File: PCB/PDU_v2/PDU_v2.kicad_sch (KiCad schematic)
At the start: 61 parts, among them J1 XT60PW-M, J14 Conn_01x04_Pin, J2 XT60PW-M, J3 XT60PW-M, J4 XT60PW-M, J5 XT60PW-M, J6 XT60PW-M, J7 XT60PW-M, U1 TPS54360BQDDAQ1, U2 INA240A2D

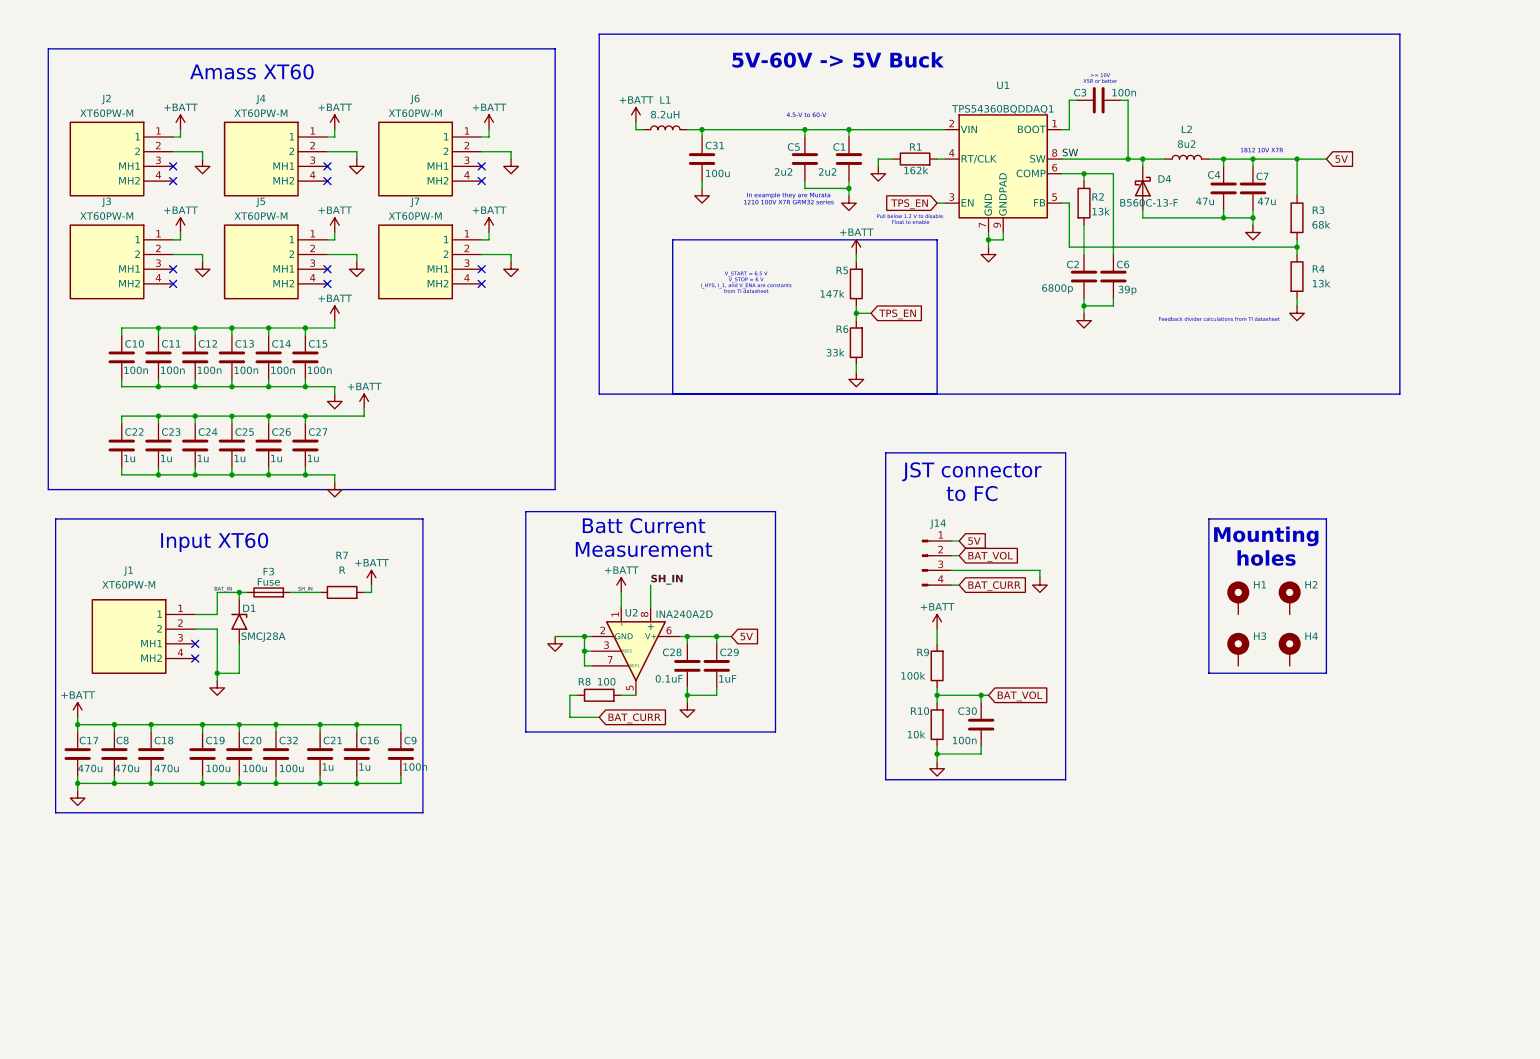
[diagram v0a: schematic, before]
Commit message: Finished layout
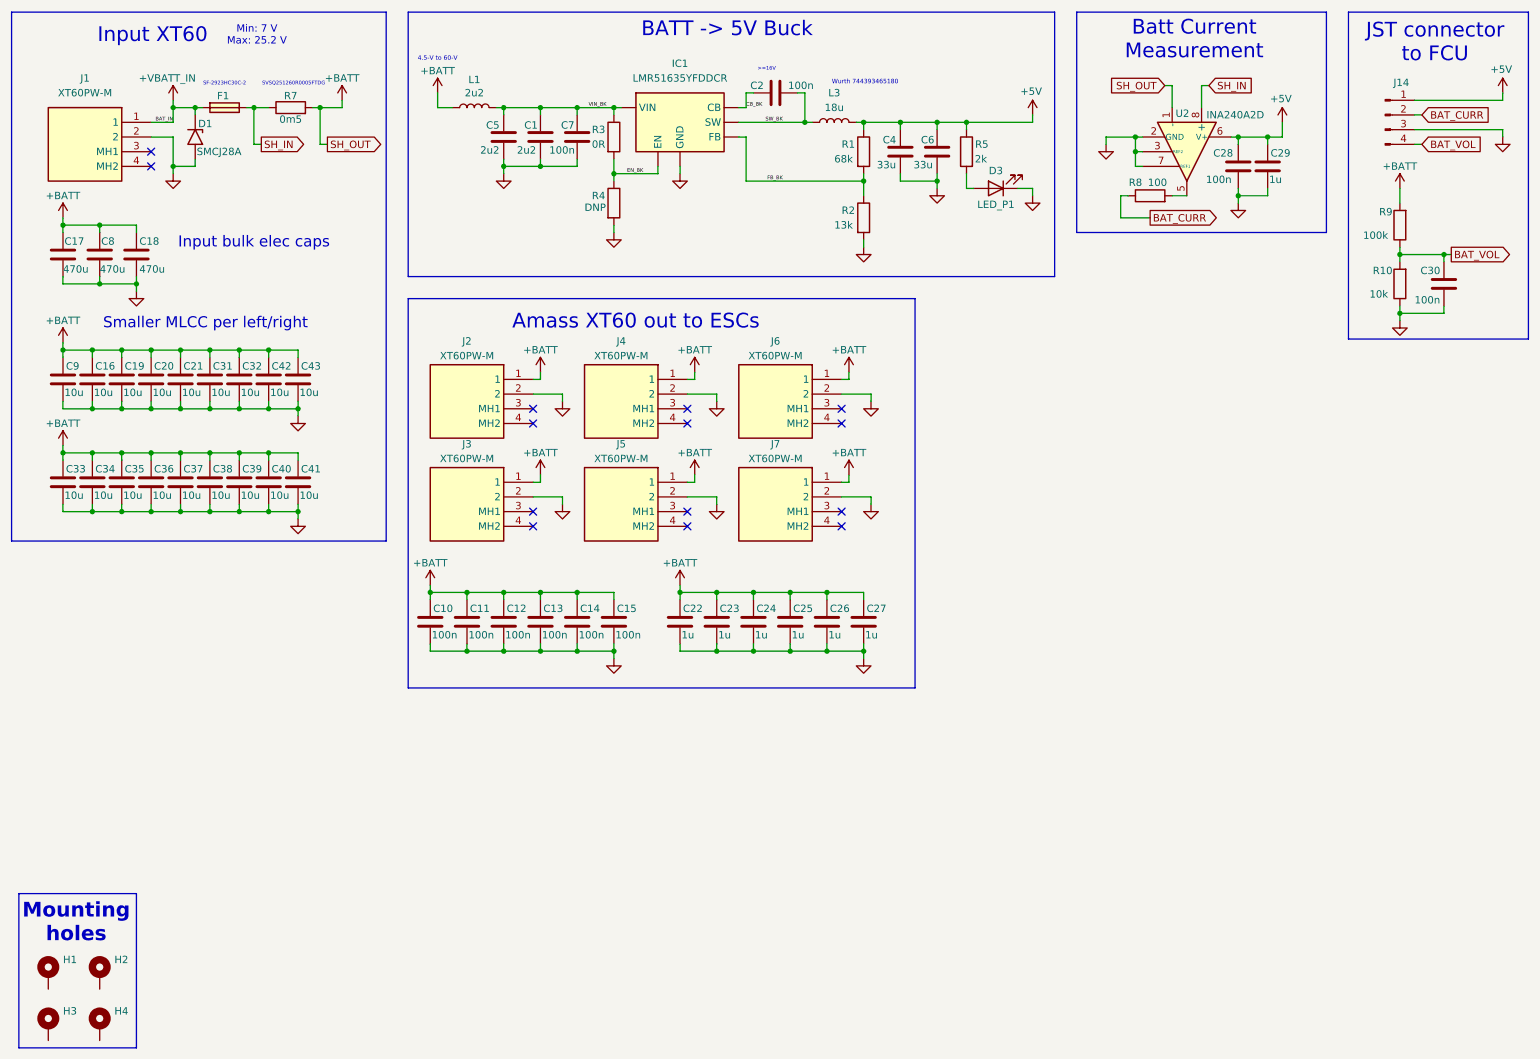
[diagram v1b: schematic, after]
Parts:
- removed C3: 100n, Capacitor_SMD:C_0805_2012Metric_Pad1.18x1.45mm_HandSolder, symbol Device:C
- removed D4: B560C-13-F, Diode_SMD:D_SMC, symbol Diode:B330
- removed F3: Fuse, Fuse:Fuse_2920_7451Metric_Pad2.10x5.45mm_HandSolder, symbol Device:Fuse
- removed L1: 8.2uH, Inductor_SMD:L_Coilcraft_XAL6060-XXX, symbol Device:L
- removed L2: 8u2, Inductor_SMD:L_Coilcraft_XAL6060-XXX, symbol Device:L
- removed R6: 33k, Resistor_SMD:R_0603_1608Metric_Pad0.98x0.95mm_HandSolder, symbol Device:R
- removed U1: TPS54360BQDDAQ1, Package_SO:TI_SO-PowerPAD-8_ThermalVias, symbol Regulator_Switching:TPS54360DDA
- added C33, C34, C35, C36, C37, C38, C39, C40, C41, C42, C43: 10u, Capacitor_SMD:C_1210_3225Metric_Pad1.33x2.70mm_HandSolder, symbol Device:C
- added D3: LED_P1, LED_SMD:LED_0805_2012Metric_Pad1.15x1.40mm_HandSolder, symbol Device:LED
- added F1: SF-2923HC30C-2, SF2923HC30C2, symbol SamacSys_Parts:SF-2923HC30C-2
- added IC1: LMR51635YFDDCR, SOT95P280X110-6N, symbol SamacSys_Parts:LMR51635YDDCR
- added L1: 2u2, WE-MAPI_4020, symbol SamacSys_Parts:74438356022
- added L3: 18u, Inductor_SMD:L_Coilcraft_XAL6060-XXX, symbol Device:L
- C16, C21: value 1u -> 10u; footprint Capacitor_SMD:C_0805_2012Metric_Pad1.18x1.45mm_HandSolder -> Capacitor_SMD:C_1210_3225Metric_Pad1.33x2.70mm_HandSolder
- C19, C20, C31, C32: value 100u -> 10u; footprint Capacitor_SMD:CP_Elec_8x10 -> Capacitor_SMD:C_1210_3225Metric_Pad1.33x2.70mm_HandSolder
- C2: value 6800p -> 100n
- C28: value 0.1uF -> 100n; footprint Capacitor_SMD:C_0805_2012Metric_Pad1.18x1.45mm_HandSolder -> Capacitor_SMD:C_0603_1608Metric_Pad1.08x0.95mm_HandSolder
- C29: value 1uF -> 1u
- C4: value 47u -> 33u; footprint Capacitor_SMD:C_0805_2012Metric_Pad1.18x1.45mm_HandSolder -> Capacitor_SMD:C_1210_3225Metric_Pad1.33x2.70mm_HandSolder
- C6: value 39p -> 33u; footprint Capacitor_SMD:C_0805_2012Metric_Pad1.18x1.45mm_HandSolder -> Capacitor_SMD:C_1210_3225Metric_Pad1.33x2.70mm_HandSolder
- C7: value 47u -> 100n
- C9: value 100n -> 10u; footprint Capacitor_SMD:C_0805_2012Metric_Pad1.18x1.45mm_HandSolder -> Capacitor_SMD:C_1210_3225Metric_Pad1.33x2.70mm_HandSolder
- R1: value 162k -> 68k
- R3: value 68k -> 0R
- R4: value 13k -> DNP
- R5: value 147k -> 2k
- R7: value R -> 0m5; footprint Resistor_SMD:R_Shunt_Vishay_WSR2_WSR3 -> Resistor_SMD:R_2512_6332Metric_Pad1.40x3.35mm_HandSolder
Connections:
- net TPS_EN is gone; now on net +5V: R5.1
- net +BATT: now also C19.2, C20.2, C31.2, C32.2, C33.2, C34.2, C35.2, C36.2, C37.2, C38.2, C39.2, C40.2, C41.2, C42.2, C43.2, L1.1; no longer C19.1, C20.1, C32.1, R5.2
- net BAT_CURR: now also J14.2 (Pin_2); no longer J14.4 (Pin_4)
- net BAT_VOL: now also J14.4 (Pin_4); no longer J14.2 (Pin_2)
- net GND: now also C19.1, C20.1, C31.1, C32.1, R2.2, C33.1, C34.1, C35.1, C36.1, C37.1, C38.1, C39.1, C40.1, C41.1, C42.1, C43.1, D3.1 (K), IC1.4 (GND); no longer C19.2, C2.2, C20.2, C31.2, C32.2, R1.1
- net SH_IN: now also F1.2
- net +5V: now reaches C6.1
- net +5V: now also C28.2, C29.2, C4.1, J14.1 (Pin_1), R1.1, U2.6 (V+), L3.2; no longer R2.1
- net VIN_BK: now reaches C1.1, C5.1
- net VIN_BK: now also C7.1, R3.1, IC1.3 (VIN), L1.2; no longer C31.1
- net CB_BK: now reaches C2.1
- net CB_BK: now also IC1.6 (CB); no longer R2.2
- net FB_BK: now reaches R1.2
- net FB_BK: now also R2.1, IC1.1 (FB)
- net EN_BK: now reaches R3.2, R4.1
- net EN_BK: now also IC1.2 (EN)
- removed net 5V: C28.2, C29.2, C4.1, C7.1, J14.1 (Pin_1), R3.1, U2.6 (V+)
- net BAT_IN renamed +VBATT_IN
- net +VBATT_IN: now also F1.1
- new net: D3.2 (A), R5.2
- new net SW_BK: C2.2, IC1.5 (SW), L3.1
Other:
- note added: ">=16V"
- note added: "Amass XT60 out to ESCs"
- note added: "BATT -> 5V Buck"
- note added: "Input bulk elec caps"
- note added: "JST connector to FCU"
- note added: "Min: 7 V Max: 25.2 V"
- note added: "SF-2923HC30C-2"
- note added: "SVSQ251260R0005FTDG"
- note added: "Smaller MLCC per left/right"
- note added: "Wurth 744393465180"
- note removed: "1812 10V X7R"
- note removed: "5V-60V -> 5V Buck"
- note removed: ">= 10V X5R or better"
- note removed: "Amass XT60"
- note removed: "Feedback divider calculations from TI datasheet"
- note removed: "In example they are Murata 1210 100V X7R GRM32 series"
- note removed: "JST connector to FC"
- note removed: "Pull below 1.2 V to disable. Float to enable"
- note removed: "V_START = 6.5 V V_STOP = 6 V I_HYS, I_1, and V_ENA are constants from TI datasheet"
- moved on the sheet: C1, C10, C11, C12, C13, C14, C15, C17, C18, C22, C23, C24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
